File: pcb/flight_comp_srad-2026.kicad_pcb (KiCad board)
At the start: 2 copper layers, 70 x 40 mm, 39 parts, among them J1 503398-1892, J2 Conn_01x04_Pin, J3 Conn_01x16_Pin, J4 Conn_01x08_Pin, J5 Conn_01x13_Pin, U1 ADXL375BCCZ-RL7, U2 MS5607-02BA, U3 RP2040, U4 NCP1117-3.3_SOT223, U5 MAX-M10M-00B, U6 W25Q128JVS, U7 IIM-20670, Y1 Crystal

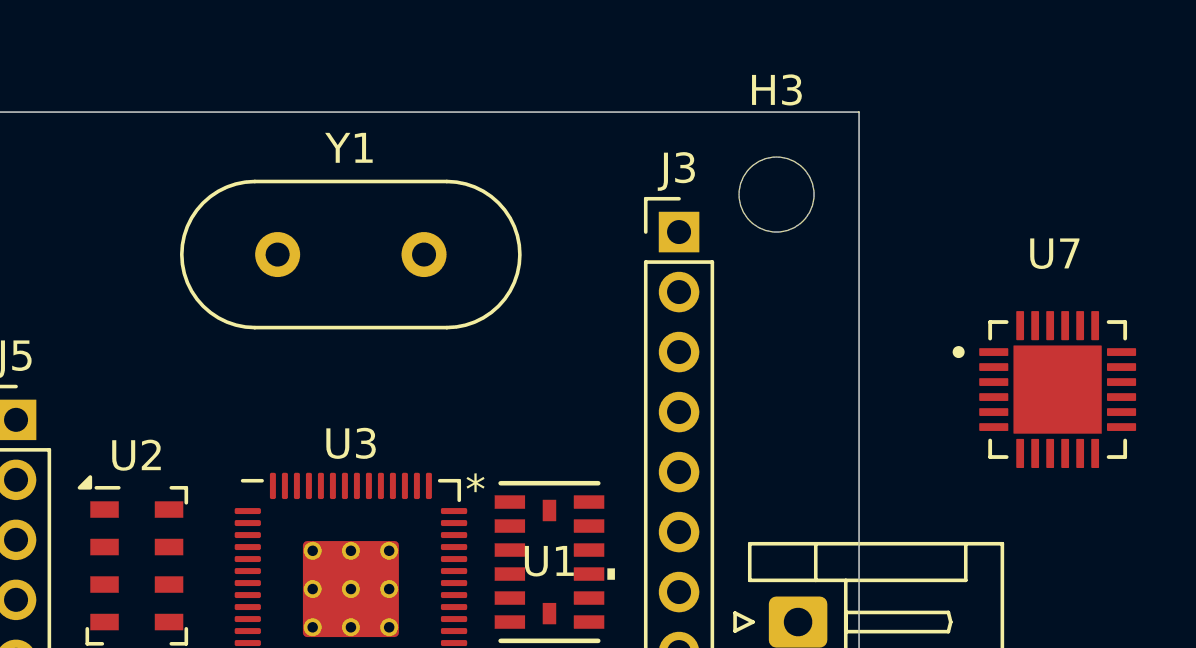
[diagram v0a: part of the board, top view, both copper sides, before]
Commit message: xtal smd
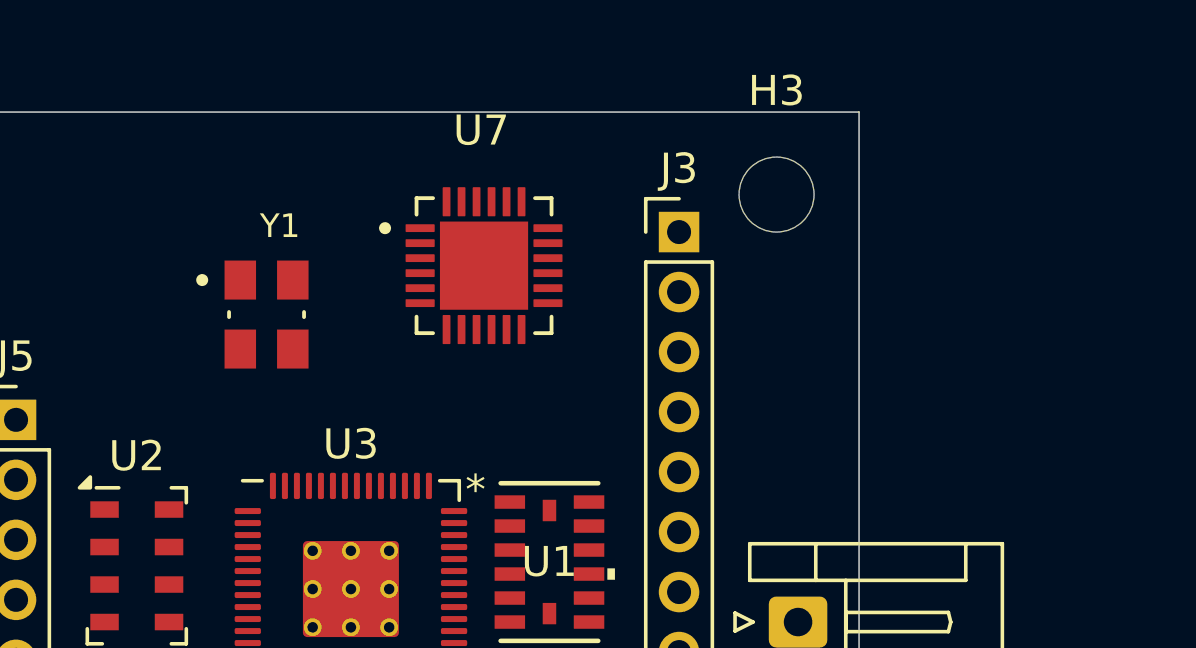
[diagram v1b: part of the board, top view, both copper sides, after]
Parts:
- Y1: value Crystal -> ABM8-272-T3; footprint Crystal:Crystal_HC49-4H_Vertical -> ABM8_272_T3:XTAL_ABM8-272-T3
- moved U7 19.6 mm to (207.5, 65.6)
- moved Y1 2.03 mm to (200.2, 67.2)
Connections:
- Y1 pad 1: Net-(C2-Pad2) -> /XIN
- Y1 pad 2: /XIN -> GND
